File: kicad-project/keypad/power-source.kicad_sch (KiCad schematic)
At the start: 20 parts, among them IC1 TPS61023DRLT, J1 Screw_Terminal_01x02, U15 MCP73832-2-OT, U2 TLV75901PDRVT

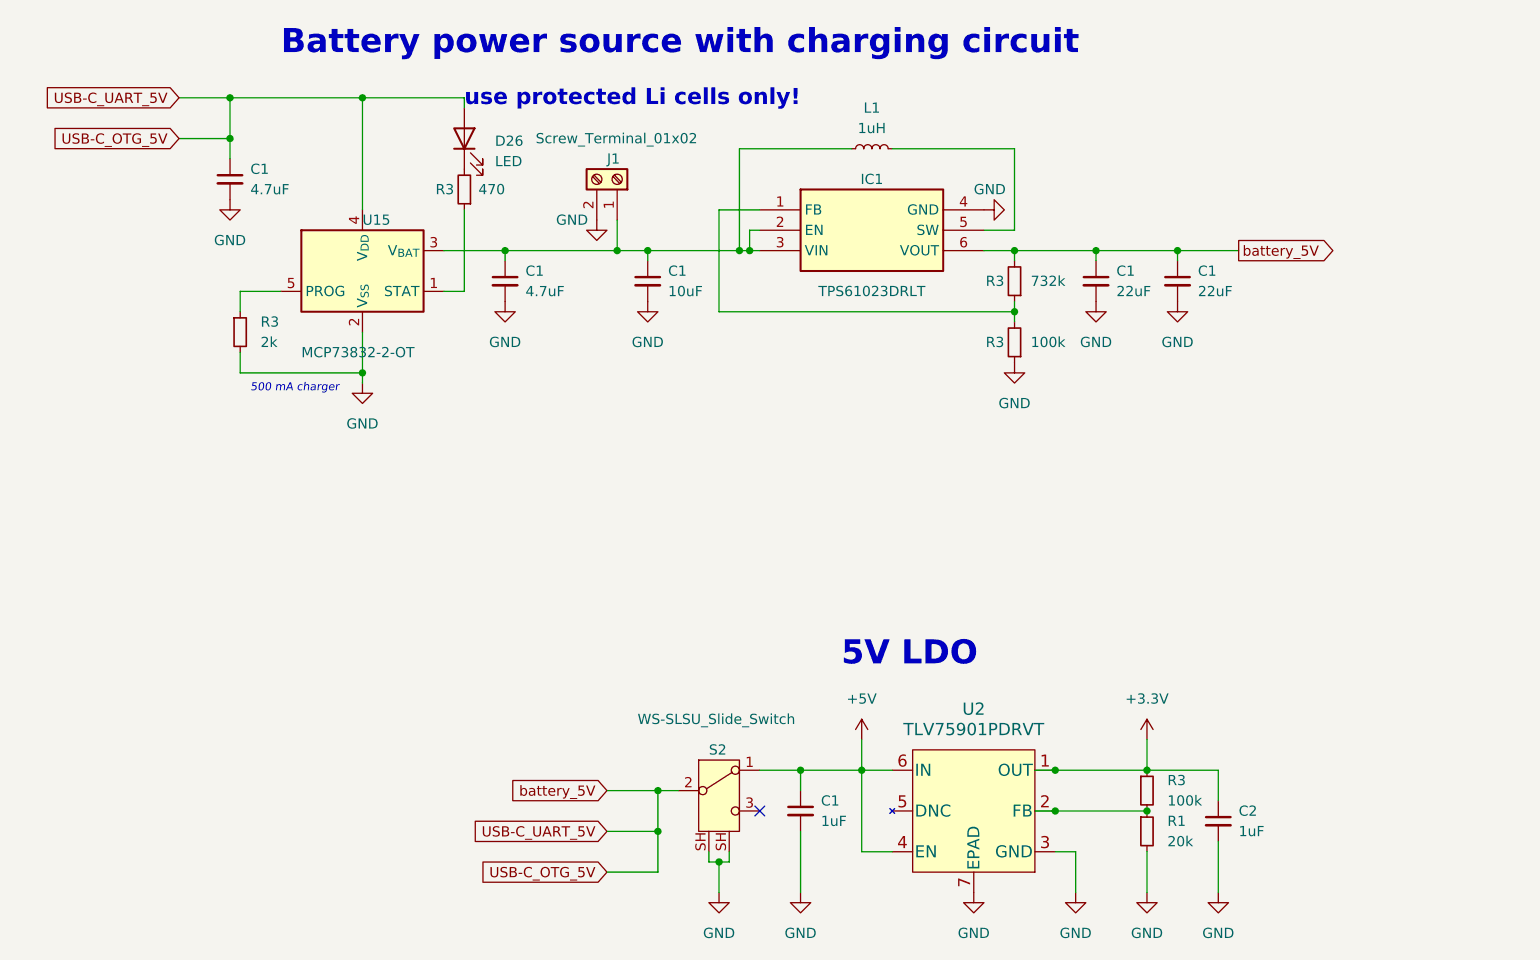
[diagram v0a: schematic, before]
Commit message: update project
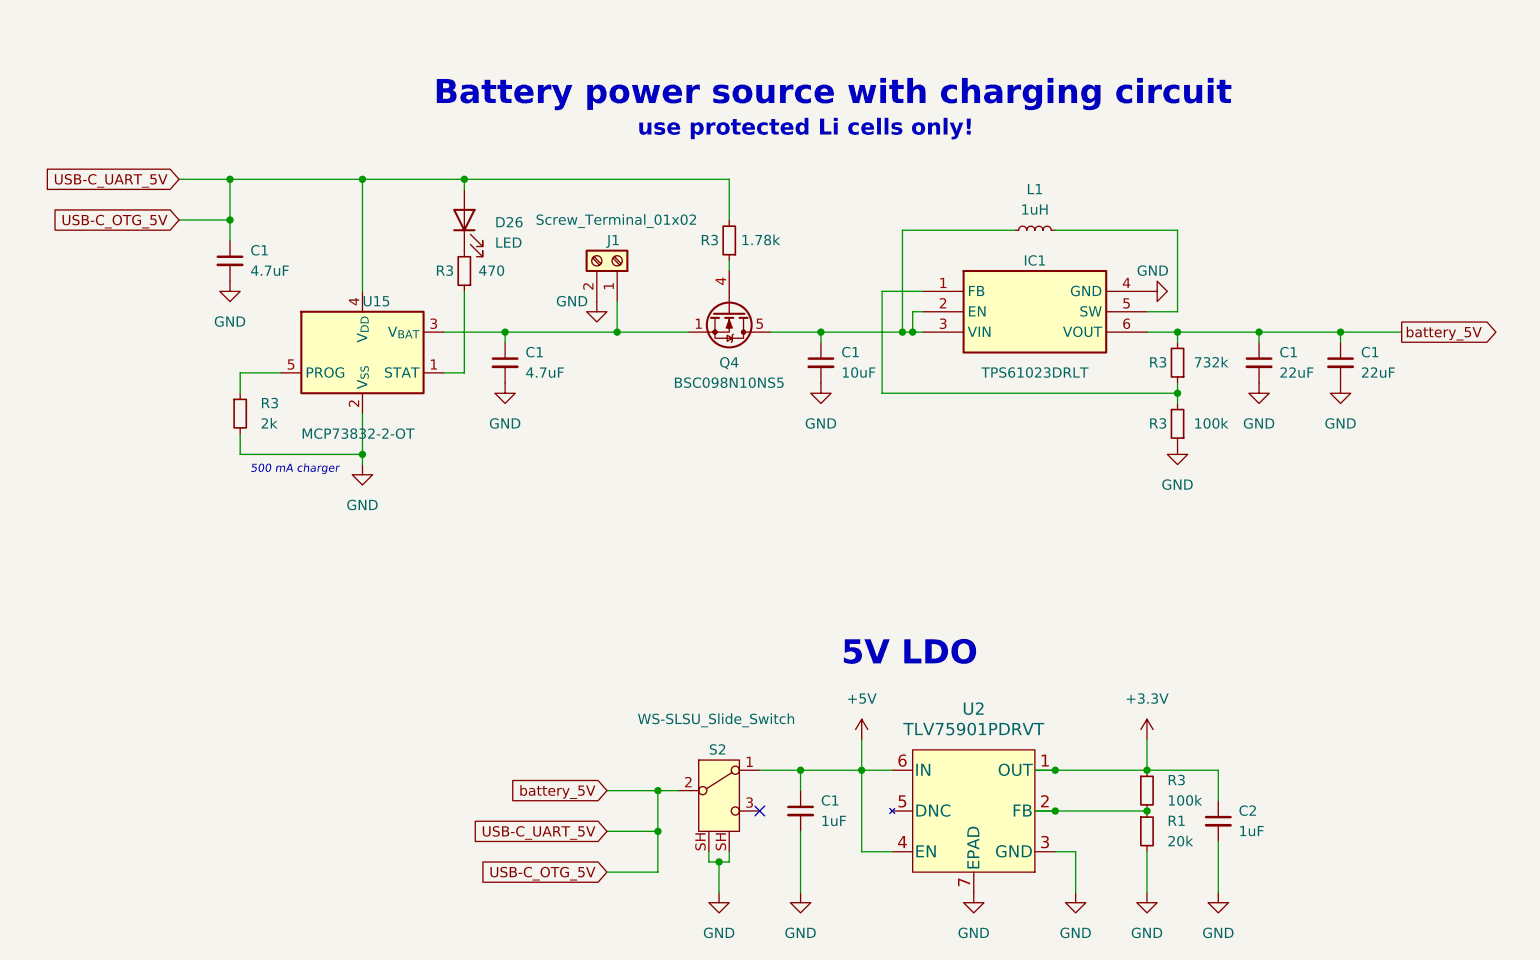
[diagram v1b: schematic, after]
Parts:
- added Q4: BSC098N10NS5, Package_TO_SOT_SMD:TDSON-8-1, symbol Transistor_FET:BSC098N10NS5
- added R3: 1.78k, Resistor_SMD:R_0603_1608Metric, symbol PutRocketLab_RCL:R_Small
- L1: footprint Inductor_SMD:L_Bourns_SRP1038C_10.0x10.0mm -> PUT_RocketLab_IC:INDPM5752X200N
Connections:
- net USB-C_OTG_5V: now also R3.2
- net at C1.1, IC1.2 (EN), IC1.3 (VIN)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: now also Q4.5 (D); no longer C1.1, J1.1 (Pin_1), U15.3 (V_{BAT})
- new net: C1.1, J1.1 (Pin_1), Q4.1 (S), Q4.2 (S), Q4.3 (S), U15.3 (V_{BAT})
- new net: Q4.4 (G), R3.1
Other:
- moved on the sheet: C1, D26, IC1, J1, L1, R3, U15

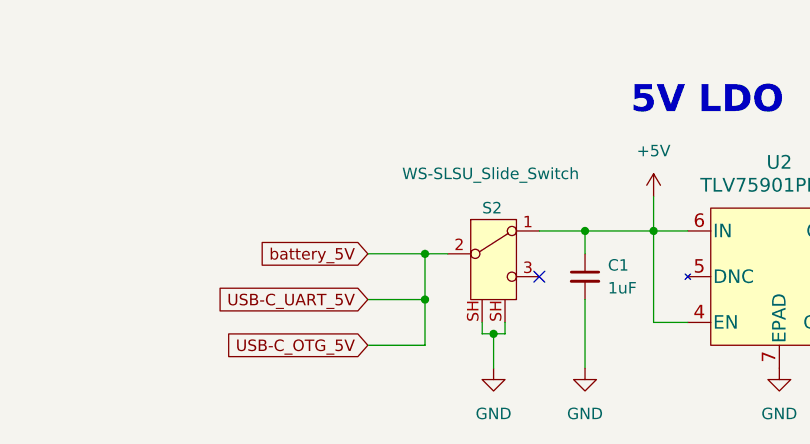
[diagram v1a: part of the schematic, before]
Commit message: correct schematic
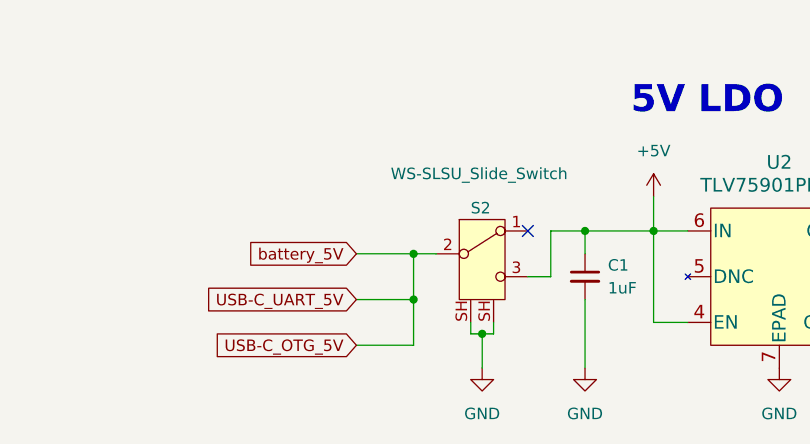
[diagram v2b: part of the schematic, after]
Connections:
- net +5V: now also S2.3; no longer S2.1
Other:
- moved on the sheet: S2
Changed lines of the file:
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@@
   (junction (at 138.43 120.65) (diameter 0) (color 0 0 0 0)
   )
-  (junction (at 120.65 132.08) (diameter 0) (color 0 0 0 0)
+  (junction (at 119.38 132.08) (diameter 0) (color 0 0 0 0)
   )
   (junction (at 187.96 66.04) (diameter 0) (color 0 0 0 0)
@@
   (junction (at 76.2 46.99) (diameter 0) (color 0 0 0 0)
   )
+  (junction (at 130.81 120.65) (diameter 0) (color 0 0 0 0)
+  )
   (junction (at 177.8 73.66) (diameter 0) (color 0 0 0 0)
   )
@@
   (junction (at 59.69 46.99) (diameter 0) (color 0 0 0 0)
   )
-  (junction (at 113.03 128.27) (diameter 0) (color 0 0 0 0)
-  )
-  (junction (at 113.03 123.19) (diameter 0) (color 0 0 0 0)
-  )
-  (junction (at 130.81 120.65) (diameter 0) (color 0 0 0 0)
+  (junction (at 111.76 128.27) (diameter 0) (color 0 0 0 0)
+  )
+  (junction (at 111.76 123.19) (diameter 0) (color 0 0 0 0)
   )
   (junction (at 76.2 81.28) (diameter 0) (color 0 0 0 0)
@@
   (junction (at 133.35 66.04) (diameter 0) (color 0 0 0 0)
   )
-  (no_connect (at 125.73 125.73))
+  (no_connect (at 124.46 120.65))
   (wire (pts (xy 146.05 60.96) (xy 140.97 60.96))
     (stroke (width 0) (type default))
@@
     (stroke (width 0) (type default))
   )
-  (wire (pts (xy 106.68 133.35) (xy 113.03 133.35))
+  (wire (pts (xy 105.41 133.35) (xy 111.76 133.35))
     (stroke (width 0) (type default))
   )
@@
     (stroke (width 0) (type default))
   )
-  (wire (pts (xy 125.73 120.65) (xy 130.81 120.65))
-    (stroke (width 0) (type default))
-  )
   (wire (pts (xy 143.51 66.04) (xy 144.78 66.04))
     (stroke (width 0) (type default))
@@
     (stroke (width 0) (type default))
   )
+  (wire (pts (xy 124.46 125.73) (xy 127 125.73))
+    (stroke (width 0) (type default))
+  )
   (wire (pts (xy 143.51 53.34) (xy 143.51 66.04))
     (stroke (width 0) (type default))
   )
-  (wire (pts (xy 121.92 132.08) (xy 120.65 132.08))
+  (wire (pts (xy 120.65 132.08) (xy 119.38 132.08))
     (stroke (width 0) (type default))
   )
@@
     (stroke (width 0) (type default))
   )
+  (wire (pts (xy 127 120.65) (xy 130.81 120.65))
+    (stroke (width 0) (type default))
+  )
   (wire (pts (xy 88.9 46.99) (xy 88.9 48.26))
     (stroke (width 0) (type default))
@@
     (stroke (width 0) (type default))
   )
-  (wire (pts (xy 119.38 132.08) (xy 119.38 130.81))
+  (wire (pts (xy 118.11 132.08) (xy 118.11 130.81))
     (stroke (width 0) (type default))
   )
@@
     (stroke (width 0) (type default))
   )
-  (wire (pts (xy 121.92 130.81) (xy 121.92 132.08))
+  (wire (pts (xy 120.65 130.81) (xy 120.65 132.08))
     (stroke (width 0) (type default))
   )
@@
     (stroke (width 0) (type default))
   )
+  (wire (pts (xy 127 125.73) (xy 127 120.65))
+    (stroke (width 0) (type default))
+  )
   (wire (pts (xy 173.99 66.04) (xy 177.8 66.04))
     (stroke (width 0) (type default))
@@
     (stroke (width 0) (type default))
   )
-  (wire (pts (xy 120.65 132.08) (xy 120.65 135.89))
-    (stroke (width 0) (type default))
-  )
-  (wire (pts (xy 106.68 123.19) (xy 113.03 123.19))
+  (wire (pts (xy 119.38 132.08) (xy 119.38 135.89))
+    (stroke (width 0) (type default))
+  )
+  (wire (pts (xy 105.41 123.19) (xy 111.76 123.19))
     (stroke (width 0) (type default))
   )
@@
     (stroke (width 0) (type default))
   )
-  (wire (pts (xy 113.03 123.19) (xy 113.03 128.27))
-    (stroke (width 0) (type default))
-  )
-  (wire (pts (xy 113.03 123.19) (xy 115.57 123.19))
-    (stroke (width 0) (type default))
-  )
-  (wire (pts (xy 113.03 133.35) (xy 113.03 128.27))
+  (wire (pts (xy 111.76 123.19) (xy 111.76 128.27))
+    (stroke (width 0) (type default))
+  )
+  (wire (pts (xy 111.76 123.19) (xy 114.3 123.19))
+    (stroke (width 0) (type default))
+  )
+  (wire (pts (xy 111.76 133.35) (xy 111.76 128.27))
     (stroke (width 0) (type default))
   )
@@
     (stroke (width 0) (type default))
   )
-  (wire (pts (xy 120.65 132.08) (xy 119.38 132.08))
-    (stroke (width 0) (type default))
-  )
-  (wire (pts (xy 106.68 128.27) (xy 113.03 128.27))
+  (wire (pts (xy 119.38 132.08) (xy 118.11 132.08))
+    (stroke (width 0) (type default))
+  )
+  (wire (pts (xy 105.41 128.27) (xy 111.76 128.27))
     (stroke (width 0) (type default))
   )
@@
     )
   )
-  (global_label "USB-C_OTG_5V" (shape input) (at 106.68 133.35 180) (fields_autoplaced)
+  (global_label "USB-C_OTG_5V" (shape input) (at 105.41 133.35 180) (fields_autoplaced)
     (effects (font (size 1.27 1.27)) (justify right))
-    (property "Intersheetrefs" "${INTERSHEET_REFS}" (at 89.241 133.35 0)
+    (property "Intersheetrefs" "${INTERSHEET_REFS}" (at 87.971 133.35 0)
       (effects (font (size 1.27 1.27)) (justify right) hide)
     )
   )
-  (global_label "battery_5V" (shape input) (at 106.68 123.19 180) (fields_autoplaced)
+  (global_label "battery_5V" (shape input) (at 105.41 123.19 180) (fields_autoplaced)
     (effects (font (size 1.27 1.27)) (justify right))
-    (property "Intersheetrefs" "${INTERSHEET_REFS}" (at 93.8373 123.19 0)
+    (property "Intersheetrefs" "${INTERSHEET_REFS}" (at 92.5673 123.19 0)
       (effects (font (size 1.27 1.27)) (justify right) hide)
     )
   )
-  (global_label "USB-C_UART_5V" (shape input) (at 106.68 128.27 180) (fields_autoplaced)
+  (global_label "USB-C_UART_5V" (shape input) (at 105.41 128.27 180) (fields_autoplaced)
     (effects (font (size 1.27 1.27)) (justify right))
-    (property "Intersheetrefs" "${INTERSHEET_REFS}" (at 88.1524 128.27 0)
+    (property "Intersheetrefs" "${INTERSHEET_REFS}" (at 86.8824 128.27 0)
       (effects (font (size 1.27 1.27)) (justify right) hide)
     )
@@
     )
   )
-  (symbol (lib_id "PUTRocketLab_supply:GND") (at 120.65 135.89 0) (unit 1)
-    (in_bom yes) (on_board yes) (dnp no) (fields_autoplaced)
-    (property "Reference" "#PWR05" (at 120.65 142.24 0)
-      (effects (font (size 1.27 1.27)) hide)
-    )
-    (property "Value" "GND" (at 120.65 140.97 0)
-      (effects (font (size 1.27 1.27)))
-    )
-    (property "Footprint" "" (at 120.65 135.89 0)
-      (effects (font (size 1.27 1.27)) hide)
-    )
-    (property "Datasheet" "" (at 120.65 135.89 0)
+  (symbol (lib_id "PUTRocketLab_supply:GND") (at 119.38 135.89 0) (unit 1)
+    (in_bom yes) (on_board yes) (dnp no) (fields_autoplaced)
+    (property "Reference" "#PWR05" (at 119.38 142.24 0)
+      (effects (font (size 1.27 1.27)) hide)
+    )
+    (property "Value" "GND" (at 119.38 140.97 0)
+      (effects (font (size 1.27 1.27)))
+    )
+    (property "Footprint" "" (at 119.38 135.89 0)
+      (effects (font (size 1.27 1.27)) hide)
+    )
+    (property "Datasheet" "" (at 119.38 135.89 0)
       (effects (font (size 1.27 1.27)) hide)
     )
@@
     )
   )
-  (symbol (lib_id "PUT_RocketLab_misc:WS-SLSU_Slide_Switch") (at 120.65 123.19 0) (unit 1)
+  (symbol (lib_id "PUT_RocketLab_misc:WS-SLSU_Slide_Switch") (at 119.38 123.19 0) (unit 1)
     (in_bom yes) (on_board yes) (dnp no)
-    (property "Reference" "S2" (at 119.38 118.11 0)
-      (effects (font (size 1.27 1.27)) (justify left))
-    )
-    (property "Value" "WS-SLSU_Slide_Switch" (at 110.49 114.3 0)
-      (effects (font (size 1.27 1.27)) (justify left))
-    )
-    (property "Footprint" "PUT_RocketLab_other:EG1206A" (at 120.65 123.19 0)
-      (effects (font (size 1.27 1.27)) hide)
-    )
-    (property "Datasheet" "" (at 120.65 123.19 0)
-      (effects (font (size 1.27 1.27)) hide)
-    )
+    (property "Reference" "S2" (at 118.11 118.11 0)
+      (effects (font (size 1.27 1.27)) (justify left))
+    )
+    (property "Value" "WS-SLSU_Slide_Switch" (at 109.22 114.3 0)
+      (effects (font (size 1.27 1.27)) (justify left))
+    )
+    (property "Footprint" "PUT_RocketLab_other:EG1206A" (at 119.38 123.19 0)
+      (effects (font (size 1.27 1.27)) hide)
+    )
+    (property "Datasheet" "" (at 119.38 123.19 0)
+      (effects (font (size 1.27 1.27)) hide)
+    )
